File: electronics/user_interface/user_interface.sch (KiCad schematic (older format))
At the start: 2 parts

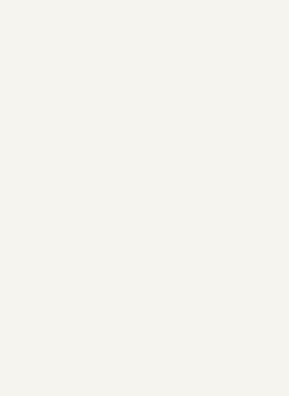
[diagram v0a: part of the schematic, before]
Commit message: started with user interface schematic entry
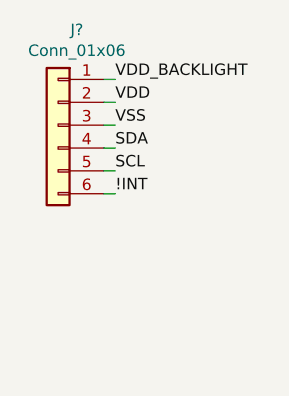
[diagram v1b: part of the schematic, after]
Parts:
- added J?: Conn_01x06, symbol Connector_Generic:Conn_01x06
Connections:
- new net !INT: J?.6 (Pin_6)
- new net SCL: J?.5 (Pin_5)
- new net SDA: J?.4 (Pin_4)
- new net VDD: J?.2 (Pin_2)
- new net VDD_BACKLIGHT: J?.1 (Pin_1)
- new net VSS: J?.3 (Pin_3)
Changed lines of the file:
@@
 EESchema Schematic File Version 4
-LIBS:jlcpcb_2_layer-cache
-EELAYER 26 0
+EELAYER 30 0
 EELAYER END
 $Descr A4 11693 8268
@@
 	1    0    0    -1
 $EndComp
+$Comp
+L Connector_Generic:Conn_01x06 J?
+U 1 1 5EBB1AC4
+P 700 1000
+F 0 "J?" H 618 1417 50  0000 C CNN
+F 1 "Conn_01x06" H 618 1326 50  0000 C CNN
+F 2 "" H 700 1000 50  0001 C CNN
+F 3 "~" H 700 1000 50  0001 C CNN
+	1    700  1000
+	-1   0    0    -1
+$EndComp
+Text Label 950  1000 0    50   ~ 0
+VSS
+Text Label 950  900  0    50   ~ 0
+VDD
+Text Label 950  800  0    50   ~ 0
+VDD_BACKLIGHT
+Text Label 950  1100 0    50   ~ 0
+SDA
+Text Label 950  1200 0    50   ~ 0
+SCL
+Text Label 950  1300 0    50   ~ 0
+!INT
+Wire Wire Line
+	900  800  950  800
+Wire Wire Line
+	950  900  900  900
+Wire Wire Line
+	900  1000 950  1000
+Wire Wire Line
+	950  1100 900  1100
+Wire Wire Line
+	900  1200 950  1200
+Wire Wire Line
+	950  1300 900  1300
 $EndSCHEMATC
